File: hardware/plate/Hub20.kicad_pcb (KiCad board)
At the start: 4 copper layers, 84.2 x 118.2 mm, 4 parts

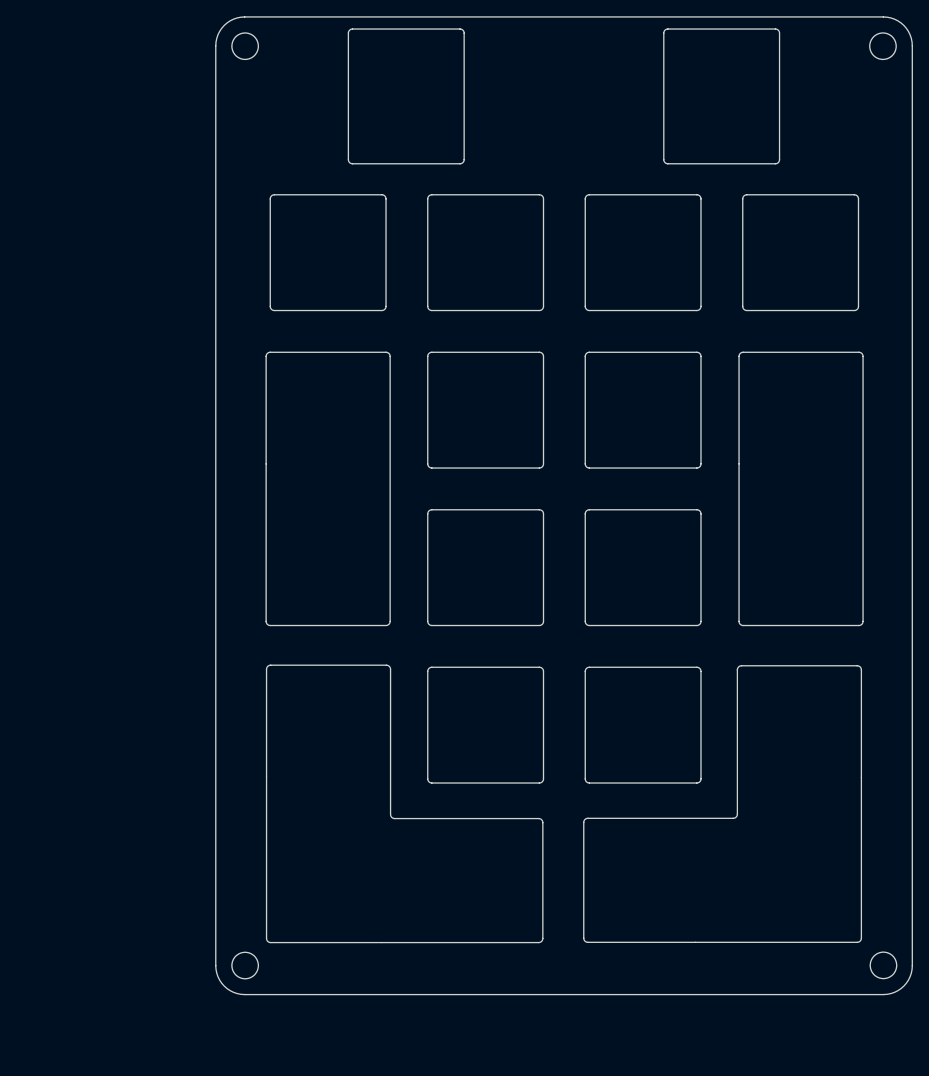
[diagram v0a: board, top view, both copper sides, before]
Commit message: center encoders :/
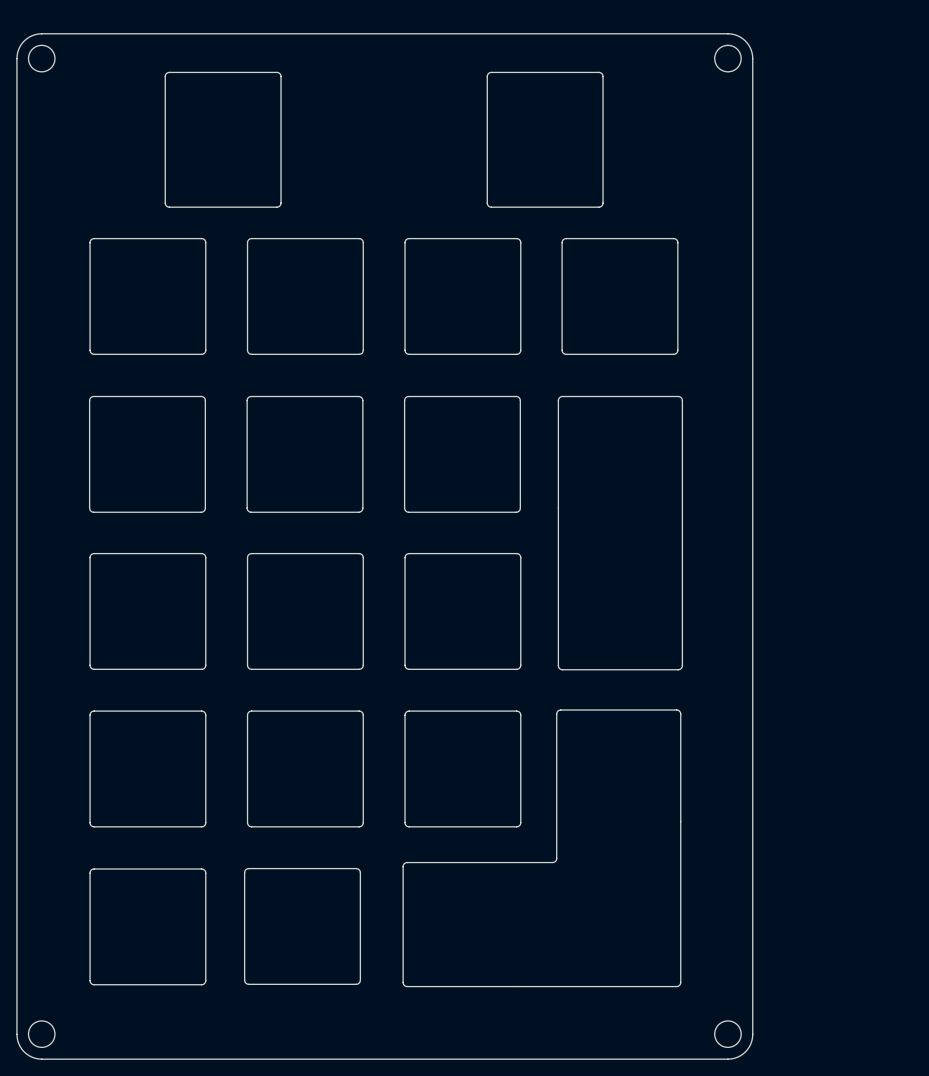
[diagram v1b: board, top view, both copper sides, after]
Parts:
- moved H4 26.0 mm to (77.9, 158.9)
- moved H2 24.6 mm to (77.9, 40.9)
- moved H3 20.6 mm to (160.9, 158.9)
- moved H1 18.8 mm to (160.9, 40.9), turned to 90 degrees
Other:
- board size 84.2 x 118.2 mm -> 89 x 124 mm
- board text removed: "JLCJLCJLC"
